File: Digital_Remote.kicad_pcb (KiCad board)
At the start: 2 copper layers, 37 parts, among them U1 STM32F103C8Tx, U2 AS01-SPI, U3 MPU-6050, U4 MT3608, U5 AMS1117-3.3, U6 TP4056, Y1 8Mhz, Y2 32KHz

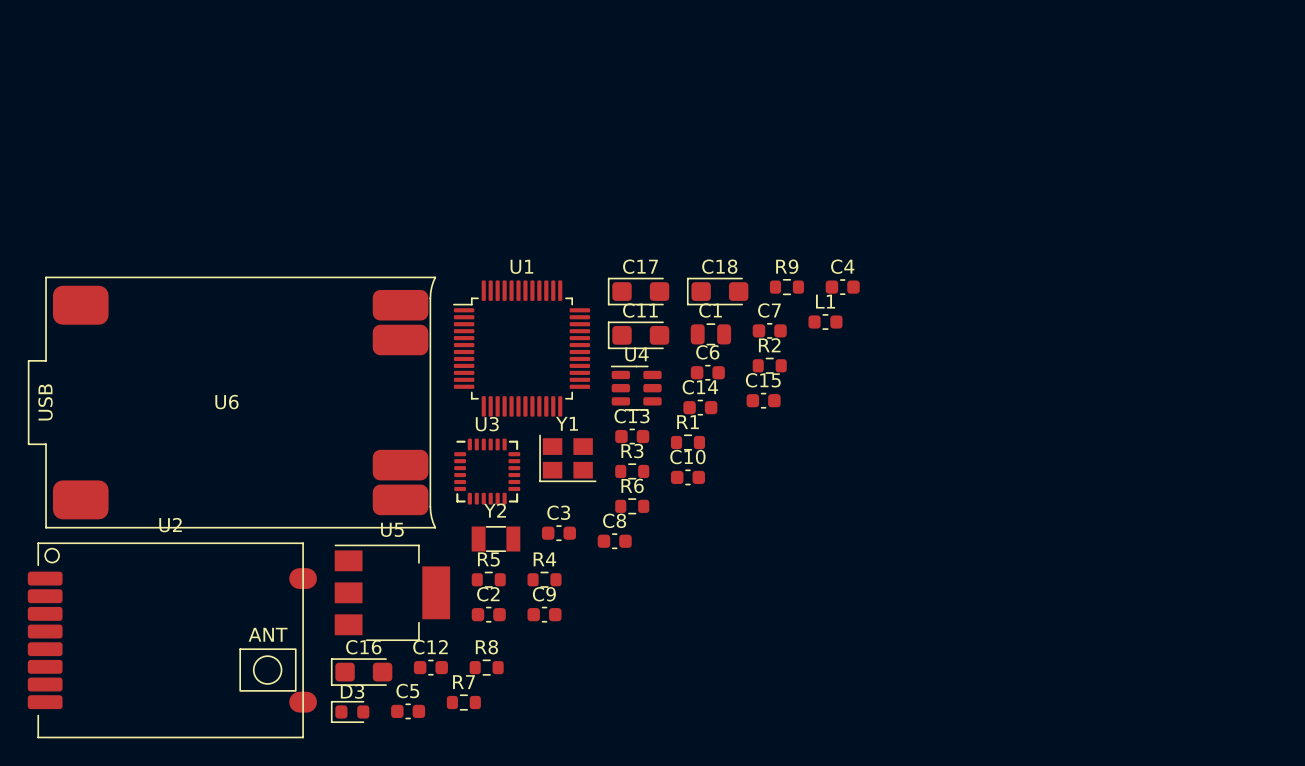
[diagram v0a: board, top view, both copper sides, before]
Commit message: Change schematic
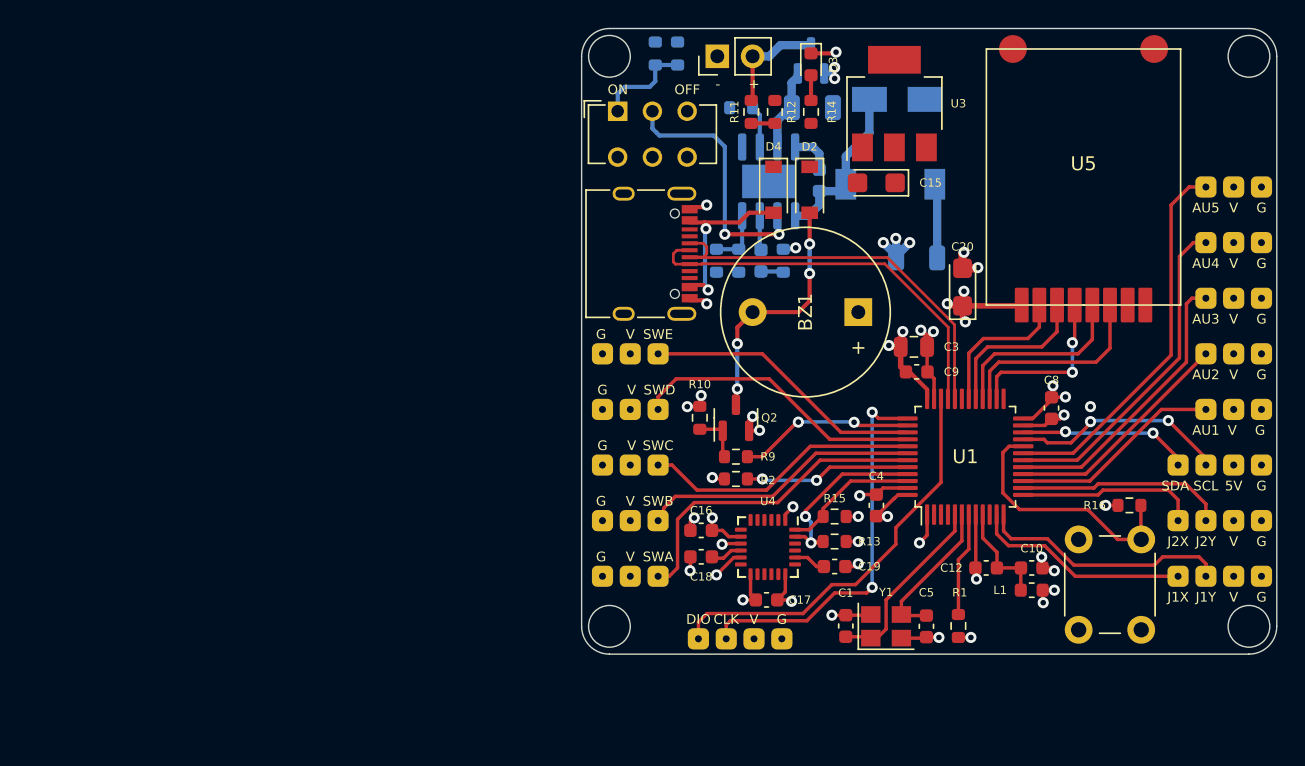
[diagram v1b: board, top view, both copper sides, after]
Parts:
- removed C2: 100n, Capacitor_SMD:C_0603_1608Metric
- removed C6: 1u, Capacitor_SMD:C_0603_1608Metric
- removed U6: TP4056, myCustomLibs:TP4056
- removed Y2: 32KHz, Crystal:Crystal_SMD_3215-2Pin_3.2x1.5mm
- added BZ1: Buzzer, Buzzer_Beeper:Buzzer_12x9.5RM7.6, F.Cu at (154.9, 80.4)
- added C19: 2.2n, Capacitor_SMD:C_0603_1608Metric, F.Cu at (153.2, 98.7)
- added C20: 22uF, Capacitor_Tantalum_SMD:CP_EIA-3216-10_Kemet-I, F.Cu at (162.4, 78.6)
- added D1: SS34, Diode_SMD:D_SMA, B.Cu at (157.7, 65.1)
- added D2: S7, Diode_SMD:D_SOD-123, F.Cu at (151.4, 71.6)
- added D4: S7, Diode_SMD:D_SOD-123, F.Cu at (148.8, 71.6)
- added J1: Conn_01x03, MyConnector:con_01x03_W2.5mm-H2.5mm, F.Cu at (181.9, 87.4)
- added J10: Conn_01x03, MyConnector:con_01x03_W2.5mm-H2.5mm, F.Cu at (181.9, 79.4)
- added J11: Conn_01x03, MyConnector:con_01x03_W2.5mm-H2.5mm, F.Cu at (181.9, 75.4)
- added J12: Conn_01x03, MyConnector:con_01x03_W2.5mm-H2.5mm, F.Cu at (181.9, 71.4)
- added J13: Conn_01x04, MyConnector:con_01x04_W2.5mm-H2.5mm, F.Cu at (180.9, 99.4)
- added J14: Conn_01x04, MyConnector:con_01x04_W2.5mm-H2.5mm, F.Cu at (180.9, 95.4)
- added J15: USB_C_Receptacle_USB2.0, Connector_USB:USB_C_Receptacle_XKB_U262-16XN-4BVC11, F.Cu at (139.1, 76.2)
- added J16: Conn_01x02, Connector_PinHeader_2.54mm:PinHeader_1x02_P2.54mm_Vertical, F.Cu at (144.8, 62.0)
- added J2: Conn_01x03, MyConnector:con_01x03_W2.5mm-H2.5mm, F.Cu at (138.5, 83.4)
- added J3: Conn_01x04, MyConnector:con_01x04_W2.5mm-H2.5mm, F.Cu at (146.4, 103.9)
- added J4: Conn_01x04, MyConnector:con_01x04_W2.5mm-H2.5mm, F.Cu at (180.9, 91.4)
- added J5: Conn_01x03, MyConnector:con_01x03_W2.5mm-H2.5mm, F.Cu at (138.5, 99.4)
- added J6: Conn_01x03, MyConnector:con_01x03_W2.5mm-H2.5mm, F.Cu at (138.5, 95.4)
- added J7: Conn_01x03, MyConnector:con_01x03_W2.5mm-H2.5mm, F.Cu at (138.5, 91.4)
- added J8: Conn_01x03, MyConnector:con_01x03_W2.5mm-H2.5mm, F.Cu at (138.5, 87.4)
- added J9: Conn_01x03, MyConnector:con_01x03_W2.5mm-H2.5mm, F.Cu at (181.9, 83.4)
- added L2: 22uH, Inductor_SMD:L_7.3x7.3_H4.5, B.Cu at (157.2, 71.2)
- added Q1: AO3401A, Package_TO_SOT_SMD:SOT-23, B.Cu at (151.5, 62.3)
- added Q2: Q_NPN_BEC, Package_TO_SOT_SMD:SOT-23, F.Cu at (146.1, 88.0)
- added R10: 10k, Resistor_SMD:R_0603_1608Metric, F.Cu at (143.5, 88.0)
- added R11: 10k, Resistor_SMD:R_0603_1608Metric, F.Cu at (147.2, 66.0)
- added R12: 3k3, Resistor_SMD:R_0603_1608Metric, F.Cu at (148.9, 66.0)
- added R13: 4k7, Resistor_SMD:R_0603_1608Metric, F.Cu at (153.2, 96.9)
- added R14: 1k, Resistor_SMD:R_0603_1608Metric, F.Cu at (151.5, 66.0)
- added R15: 4k7, Resistor_SMD:R_0603_1608Metric, F.Cu at (153.2, 95.1)
- added R16: 10k, Resistor_SMD:R_0603_1608Metric, F.Cu at (174.4, 94.3)
- added SW1: SW_SPDT, Button_Switch_THT:SW_CuK_JS202011CQN_DPDT_Straight, F.Cu at (137.6, 66.0)
- added SW2: BIND, Button_Switch_THT:SW_PUSH_6mm_H5mm, F.Cu at (175.2, 96.8)
- C1: value 4.7u -> 20p; footprint Capacitor_SMD:C_0805_2012Metric -> Capacitor_SMD:C_0603_1608Metric
- C10, C8, C9: value 20p -> 100n
- C11: value 22uF/6V -> 150pF; footprint Capacitor_Tantalum_SMD:CP_EIA-3216-10_Kemet-I -> Capacitor_SMD:C_0603_1608Metric; moved to B.Cu
- C12: value 10n -> 1u
- C13: moved to B.Cu
- C14: value 100n -> 22uF; footprint Capacitor_SMD:C_0603_1608Metric -> Capacitor_SMD:C_1206_3216Metric; moved to B.Cu
- C15: value 2.2n -> 22uF/6V; footprint Capacitor_SMD:C_0603_1608Metric -> Capacitor_Tantalum_SMD:CP_EIA-3216-10_Kemet-I
- C16: value 22uF/6V -> 10n; footprint Capacitor_Tantalum_SMD:CP_EIA-3216-10_Kemet-I -> Capacitor_SMD:C_0603_1608Metric
- C17, C18: value 22uF/6V -> 100n; footprint Capacitor_Tantalum_SMD:CP_EIA-3216-10_Kemet-I -> Capacitor_SMD:C_0603_1608Metric
- C3: value 100n -> 4.7u; footprint Capacitor_SMD:C_0603_1608Metric -> Capacitor_SMD:C_0805_2012Metric
- C5: value 100n -> 20p
- C7: value 20p -> 10uF; footprint Capacitor_SMD:C_0603_1608Metric -> Capacitor_SMD:C_1206_3216Metric; moved to B.Cu
- R3, R5: value 4k7 -> 100k; moved to B.Cu
- R4: value 4k7 -> 24k; moved to B.Cu
- R6: value 10k -> 100k; moved to B.Cu
- R7: value 24k -> 126k; moved to B.Cu
- R8: value 3k3 -> 24k; moved to B.Cu
- R9: value 1k -> 4k7
- U2: value AS01-SPI -> MP1584; footprint myCustomLibs:AS01-SPI -> Package_SO:SOIC-8-1EP_3.9x4.9mm_P1.27mm_EP2.41x3.81mm; moved to B.Cu
- U3: value MPU-6050 -> AMS1117-3.3; footprint Sensor_Motion:InvenSense_QFN-24_4x4mm_P0.5mm -> Package_TO_SOT_SMD:SOT-223-3_TabPin2
- U4: value MT3608 -> MPU-6050; footprint Package_TO_SOT_SMD:SOT-23-6 -> Sensor_Motion:InvenSense_QFN-24_4x4mm_P0.5mm
- U5: value AMS1117-3.3 -> AS01-SPI; footprint Package_TO_SOT_SMD:SOT-223-3_TabPin2 -> Wireless:AS01-SPIPX-NRF24
- moved D3 57.1 mm to (151.5, 62.6), turned to -90 degrees
- moved U2 54.6 mm to (148.4, 71.0), turned to 90 degrees
- moved U5 53.8 mm to (171.1, 79.9)
- moved C12 40.6 mm to (164.1, 98.8), turned to 180 degrees
- moved U3 39.5 mm to (157.5, 65.4), turned to 90 degrees
- moved R4 39.0 mm to (141.9, 61.8), turned to 90 degrees
- moved R5 38.5 mm to (146.5, 65.7), turned to 180 degrees
- moved C5 37.8 mm to (159.8, 103.0), turned to -90 degrees
- moved R7 37.4 mm to (146.3, 76.7), turned to 90 degrees
- moved R8 33.6 mm to (144.7, 76.7), turned to -90 degrees
- moved C8 32.8 mm to (168.8, 87.3), turned to -90 degrees
- moved U1 32.8 mm to (162.6, 90.8), turned to 90 degrees
- moved C9 32.0 mm to (159.1, 84.7)
- moved R3 30.1 mm to (140.3, 61.8), turned to -90 degrees
- moved C3 28.8 mm to (158.9, 82.9)
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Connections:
- C1 pad 1: +3V3 -> /HSE_IN
- C10 pad 1: /LSE_OUT -> +3.3VA
- C11 pad 1: +3V3 -> /COMP
- C11 pad 2: GND -> Net-(C11-Pad2)
- C12 pad 1: GND -> +3.3VA
- C12 pad 2: +3V3 -> GND
- C13 pad 1: +3V3 -> /BST
- C13 pad 2: GND -> /SW
- C14 pad 1: /REGOUT -> +5V
- C15 pad 1: /CPOUT -> +3V3
- C16 pad 1: /VIN -> GND
- C16 pad 2: GND -> +3V3
- C17 pad 1: +5V -> +3V3
- C18 pad 1: +3V3 -> /REGOUT
- C5 pad 1: +3.3VA -> /HSE_OUT
- C7 pad 1: /HSE_IN -> /VIN
- C8 pad 1: /HSE_OUT -> +3V3
- C9 pad 1: /LSE_IN -> +3V3
- R3 pad 1: +3V3 -> /VIN
- R3 pad 2: /I2C1_SCL -> Net-(R3-Pad2)
- R4 pad 1: +3V3 -> Net-(R3-Pad2)
- R4 pad 2: /I2C1_SDA -> GND
- R5 pad 1: /Buzzer -> /FREQ
- R5 pad 2: Net-(Q1-Pad1) -> GND
- R6 pad 1: GND -> Net-(C11-Pad2)
- R6 pad 2: Net-(Q1-Pad1) -> GND
- R7 pad 2: Net-(R7-Pad2) -> /FB
- R8 pad 1: Net-(R7-Pad2) -> /FB
- R9 pad 1: +3V3 -> /Buzzer
- R9 pad 2: Net-(D3-Pad2) -> Net-(Q2-Pad1)
- U1 pad 1: /VBAT -> +3V3
- U1 pad 10: unconnected-(U1-Pad10) -> /VoltageMeter
- U1 pad 11: unconnected-(U1-Pad11) -> /J1_X
- U1 pad 12: unconnected-(U1-Pad12) -> /J1_Y
- U1 pad 13: unconnected-(U1-Pad13) -> /J2_X
- U1 pad 14: /J1_X -> /J2_Y
- U1 pad 15: /J1_Y -> /AUX_1
- U1 pad 16: /J2_X -> /AUX_2
- U1 pad 17: /J2_Y -> /AUX_3
- U1 pad 18: /AUX_1 -> /AUX_4
- U1 pad 19: /AUX_2 -> /AUX_5
- U1 pad 20: unconnected-(U1-Pad20) -> /BTN_BIND
- U1 pad 21: /I2C1_SCL -> /I2C2_SCL
- U1 pad 22: unconnected-(U1-Pad22) -> /I2C2_SDA
- U1 pad 29: /NRF_CSN -> /NRF_CE
- U1 pad 3: /LSE_IN -> unconnected-(U1-Pad3)
- U1 pad 30: /NRF_CE -> /NRF_CSN
- U1 pad 32: unconnected-(U1-Pad32) -> /USB_D-
- U1 pad 33: unconnected-(U1-Pad33) -> /USB_D+
- U1 pad 34: unconnected-(U1-Pad34) -> /DIO
- U1 pad 37: unconnected-(U1-Pad37) -> /CLK
- U1 pad 39: unconnected-(U1-Pad39) -> /SWE
- U1 pad 4: /LSE_OUT -> unconnected-(U1-Pad4)
- U1 pad 40: unconnected-(U1-Pad40) -> /SWD
- U1 pad 41: unconnected-(U1-Pad41) -> /SWC
- U1 pad 42: unconnected-(U1-Pad42) -> /SWB
- U1 pad 43: unconnected-(U1-Pad43) -> /SWA
- U1 pad 45: unconnected-(U1-Pad45) -> /I2C1_SCL
- U2 pad 1: +3V3 -> /SW
- U2 pad 2: /NRF_CSN -> /EN
- U2 pad 3: /NRF_CE -> /COMP
- U2 pad 4: /SPI2_SCK -> /FB
- U2 pad 5: /SPI2_MOSI -> GND
- U2 pad 6: /SPI2_MISO -> /FREQ
- U2 pad 7: unconnected-(U2-Pad7) -> /VIN
- U2 pad 8: GND -> /BST
- U3 pad 2: (no net) -> +3V3
- U3 pad 3: (no net) -> +5V
- U4 pad 1: Net-(D2-Pad2) -> GND
- U4 pad 2: GND -> (no net)
- U4 pad 3: Net-(R7-Pad2) -> (no net)
- U4 pad 4: /EN -> (no net)
- U4 pad 5: /VIN -> (no net)
- U5 pad 1: GND -> +3V3
- U5 pad 2: +3V3 -> /NRF_CSN
- U5 pad 3: +5V -> /NRF_CE
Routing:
- net GND: track 0.00 -> 55.9 mm, vias 0 -> 33
- net +3V3: track 0.00 -> 35.6 mm, vias 0 -> 16
- net /USB_D-: track 0.00 -> 29.6 mm
- net /DIO: track 0.00 -> 29.5 mm
- net /USB_D+: track 0.00 -> 28.8 mm
- net /CLK: track 0.00 -> 27.9 mm, vias 0 -> 2
- net /AUX_5: track 0.00 -> 27.4 mm
- net /AUX_4: track 0.00 -> 23.9 mm
- net /SWA: track 0.00 -> 23.4 mm
- net /SWD: track 0.00 -> 21.2 mm
- net /AUX_3: track 0.00 -> 20.6 mm
- net /SWE: track 0.00 -> 20.3 mm
- net /SWB: track 0.00 -> 20.2 mm
- net /SWC: track 0.00 -> 20.0 mm
- net /EN: track 0.00 -> 18.6 mm, vias 0 -> 2
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- added copper zone on In2.Cu, net +3V3
- added copper zone on In1.Cu, net GND
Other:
- board outline added: 50 x 45 mm
- copper layers 2 -> 4
- board text added: "+"
- board text added: "-"
- board text added: "5V"
- board text added: "AU1"
- board text added: "AU2"
- board text added: "AU3"
- board text added: "AU4"
- board text added: "AU5"
- board text added: "CLK"
- board text added: "DIO"
- board text added: "G"
- board text added: "J1X"
- board text added: "J1Y"
- board text added: "J2X"
- board text added: "J2Y"
- board text added: "OFF"
- board text added: "ON"
- board text added: "SCL"
- board text added: "SDA"
- board text added: "SWA"
- board text added: "SWB"
- board text added: "SWC"
- board text added: "SWD"
- board text added: "SWE"
- board text added: "V"
